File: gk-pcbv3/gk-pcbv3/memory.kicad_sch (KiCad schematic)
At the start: 21 parts, among them J4 Micro_SD_Card_Det2, U6 IS42S16320F-7TLI-TR, U8 TPS2041BDBV

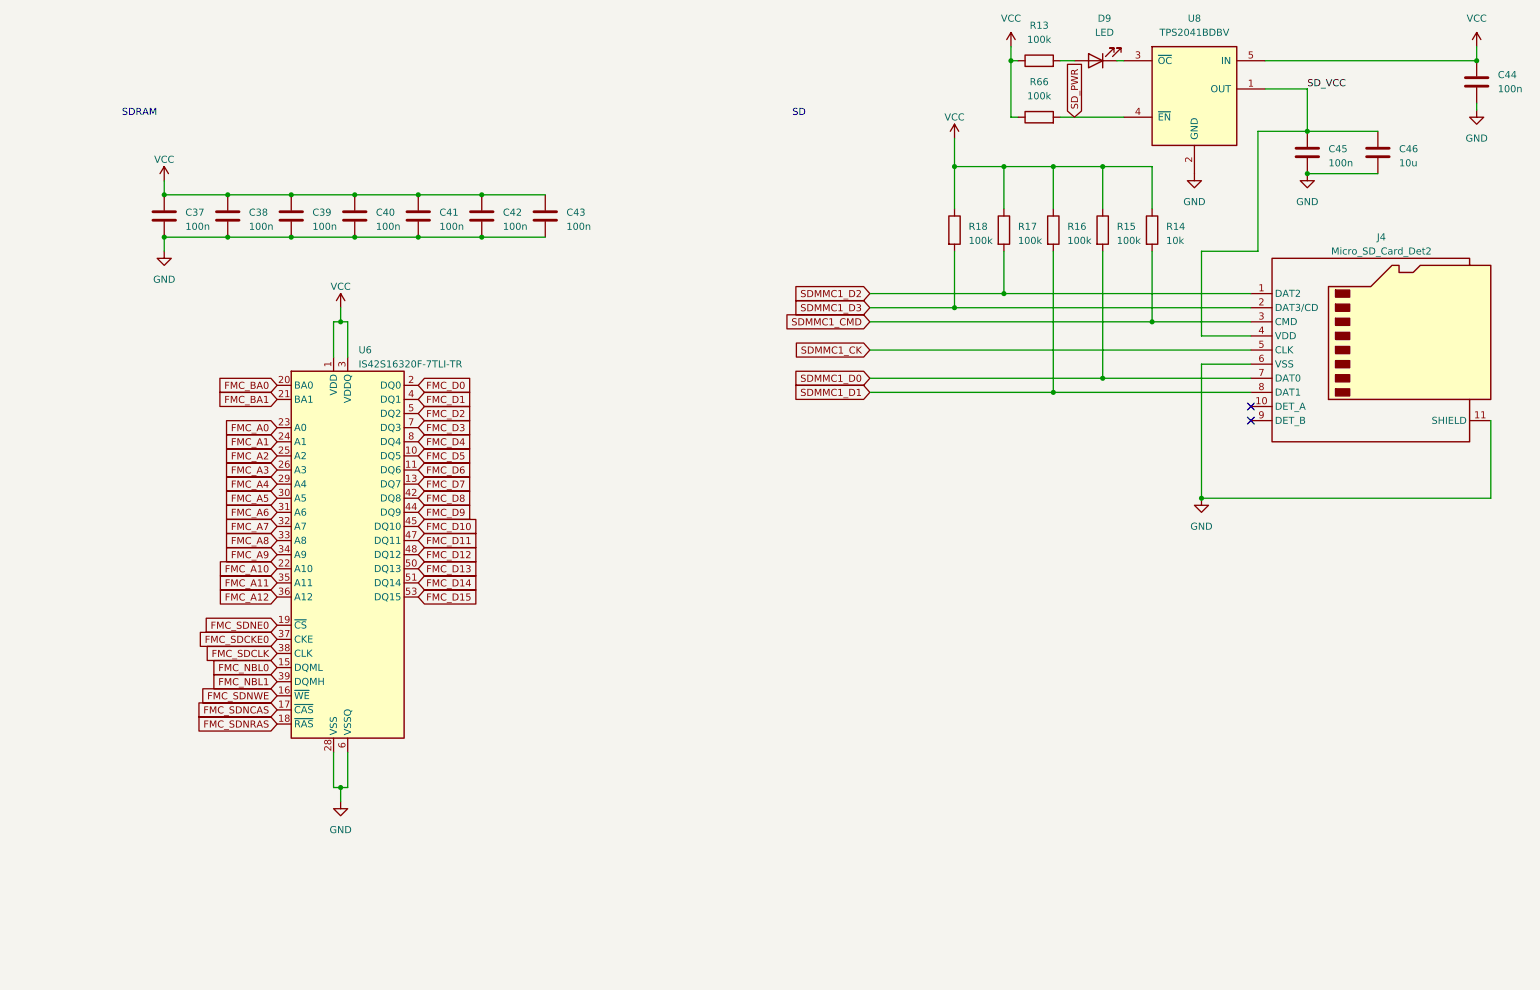
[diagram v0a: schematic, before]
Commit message: v3 board
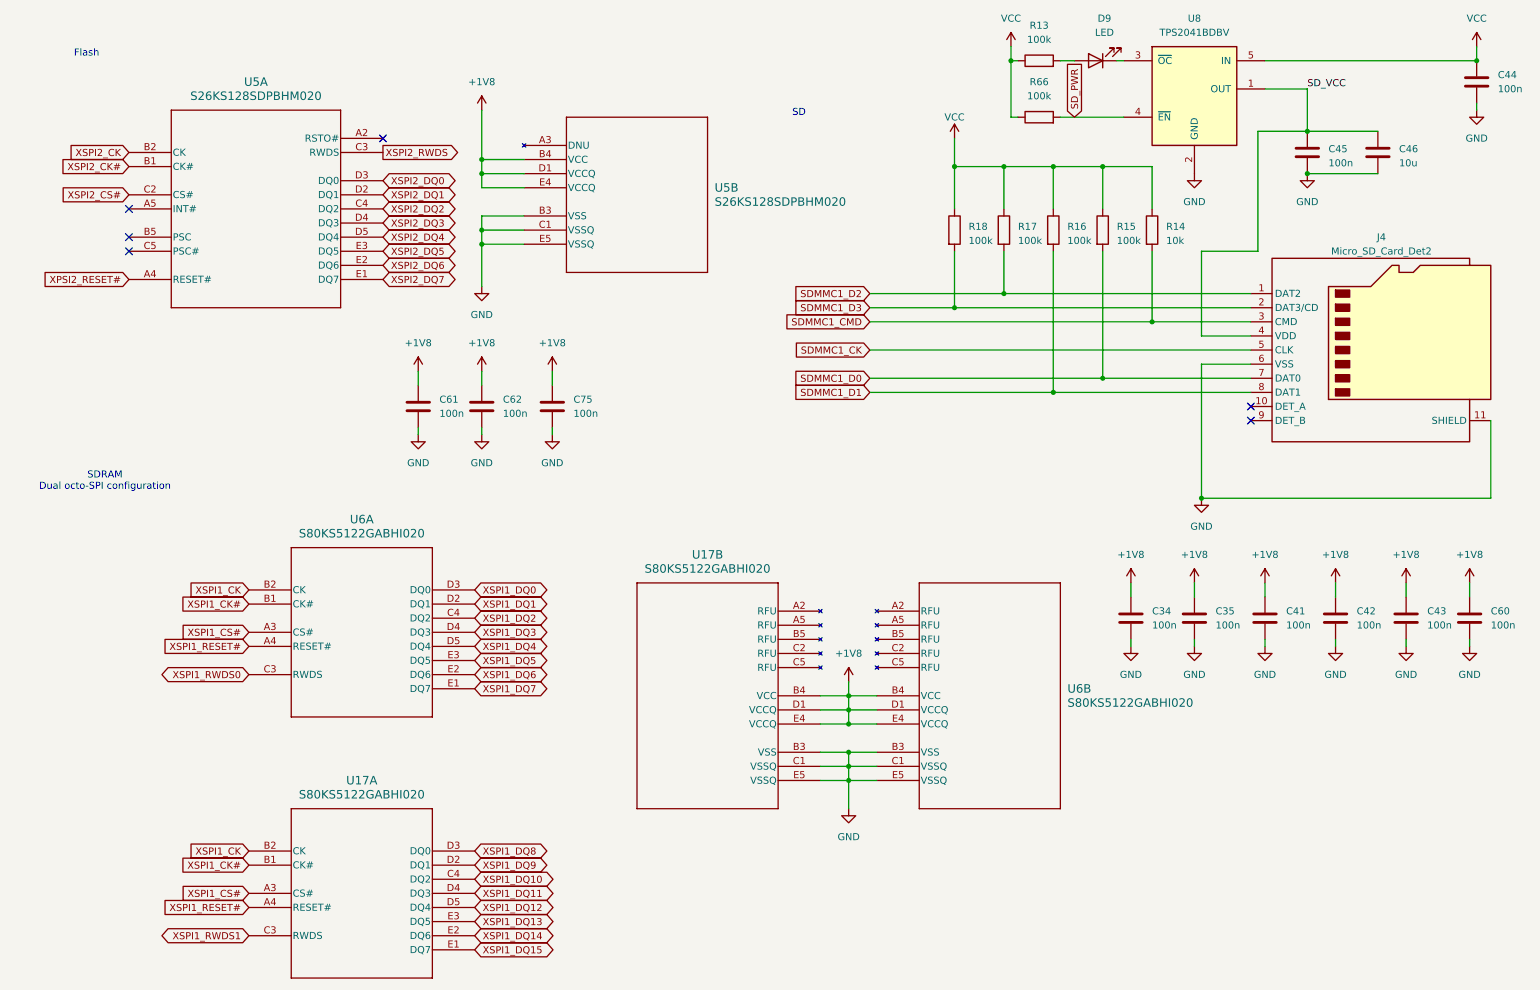
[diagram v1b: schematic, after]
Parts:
- removed C37, C38, C39, C40: 100n, Capacitor_SMD:C_0603_1608Metric, symbol Device:C
- removed U6: IS42S16320F-7TLI-TR, Package_SO:TSOP-II-54_22.2x10.16mm_P0.8mm, symbol Memory_RAM:MT48LC16M16A2P
- added C34, C35, C60, C61, C62, C75: 100n, Capacitor_SMD:C_0603_1608Metric, symbol Device:C
- added U17, U6: S80KS5122GABHI020, STM32H7S7:PG-BGA-24-801, symbol Infineon HyperRAM:S80KS5122GABHI020
- added U5: S26KS128SDPBHM020, STM32H7S7:BGA24_S26KS512SDPBHI020_CYP_INF, symbol Infineon Flash:S26KS128SDPBHM020
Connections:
- net GND: now also C34.2, C35.2, C60.2, C61.2, C62.2, C75.2, U17.B3 (VSS), U17.C1 (VSSQ), U17.E5 (VSSQ), U5.B3 (VSS), U5.C1 (VSSQ), U5.E5 (VSSQ), U6.B3 (VSS), U6.C1 (VSSQ), U6.E5 (VSSQ)
- net VCC: no longer C41.1, C42.1, C43.1
- new net +1V8: C34.1, C35.1, C41.1, C42.1, C43.1, C60.1, C61.1, C62.1, C75.1, U17.B4 (VCC), U17.D1 (VCCQ), U17.E4 (VCCQ), U5.B4 (VCC), U5.D1 (VCCQ), U5.E4 (VCCQ), U6.B4 (VCC), U6.D1 (VCCQ), U6.E4 (VCCQ)
- new net XPSI2_RESET#: U5.A4 (RESET#)
- new net XSPI1_CK: U17.B2 (CK), U6.B2 (CK)
- new net XSPI1_CK#: U17.B1 (CK#), U6.B1 (CK#)
- new net XSPI1_CS#: U17.A3 (CS#), U6.A3 (CS#)
- new net XSPI1_DQ0: U6.D3 (DQ0)
- new net XSPI1_DQ1: U6.D2 (DQ1)
- new net XSPI1_DQ10: U17.C4 (DQ2)
- new net XSPI1_DQ11: U17.D4 (DQ3)
- new net XSPI1_DQ12: U17.D5 (DQ4)
- new net XSPI1_DQ13: U17.E3 (DQ5)
- new net XSPI1_DQ14: U17.E2 (DQ6)
- new net XSPI1_DQ15: U17.E1 (DQ7)
- new net XSPI1_DQ2: U6.C4 (DQ2)
- new net XSPI1_DQ3: U6.D4 (DQ3)
- new net XSPI1_DQ4: U6.D5 (DQ4)
- new net XSPI1_DQ5: U6.E3 (DQ5)
- new net XSPI1_DQ6: U6.E2 (DQ6)
- new net XSPI1_DQ7: U6.E1 (DQ7)
- new net XSPI1_DQ8: U17.D3 (DQ0)
- new net XSPI1_DQ9: U17.D2 (DQ1)
- new net XSPI1_RESET#: U17.A4 (RESET#), U6.A4 (RESET#)
- new net XSPI1_RWDS0: U6.C3 (RWDS)
- new net XSPI1_RWDS1: U17.C3 (RWDS)
- new net XSPI2_CK: U5.B2 (CK)
- new net XSPI2_CK#: U5.B1 (CK#)
- new net XSPI2_CS#: U5.C2 (CS#)
- new net XSPI2_DQ0: U5.D3 (DQ0)
- new net XSPI2_DQ1: U5.D2 (DQ1)
- new net XSPI2_DQ2: U5.C4 (DQ2)
- new net XSPI2_DQ3: U5.D4 (DQ3)
- new net XSPI2_DQ4: U5.D5 (DQ4)
- new net XSPI2_DQ5: U5.E3 (DQ5)
- new net XSPI2_DQ6: U5.E2 (DQ6)
- new net XSPI2_DQ7: U5.E1 (DQ7)
- new net XSPI2_RWDS: U5.C3 (RWDS)
- no-connect marks 2 -> 6
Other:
- note added: "Flash"
- note added: "SDRAM Dual octo-SPI configuration"
- note removed: "SDRAM"
